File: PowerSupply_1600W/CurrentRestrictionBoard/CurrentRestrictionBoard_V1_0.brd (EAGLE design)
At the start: 160 x 100 mm, 0 parts

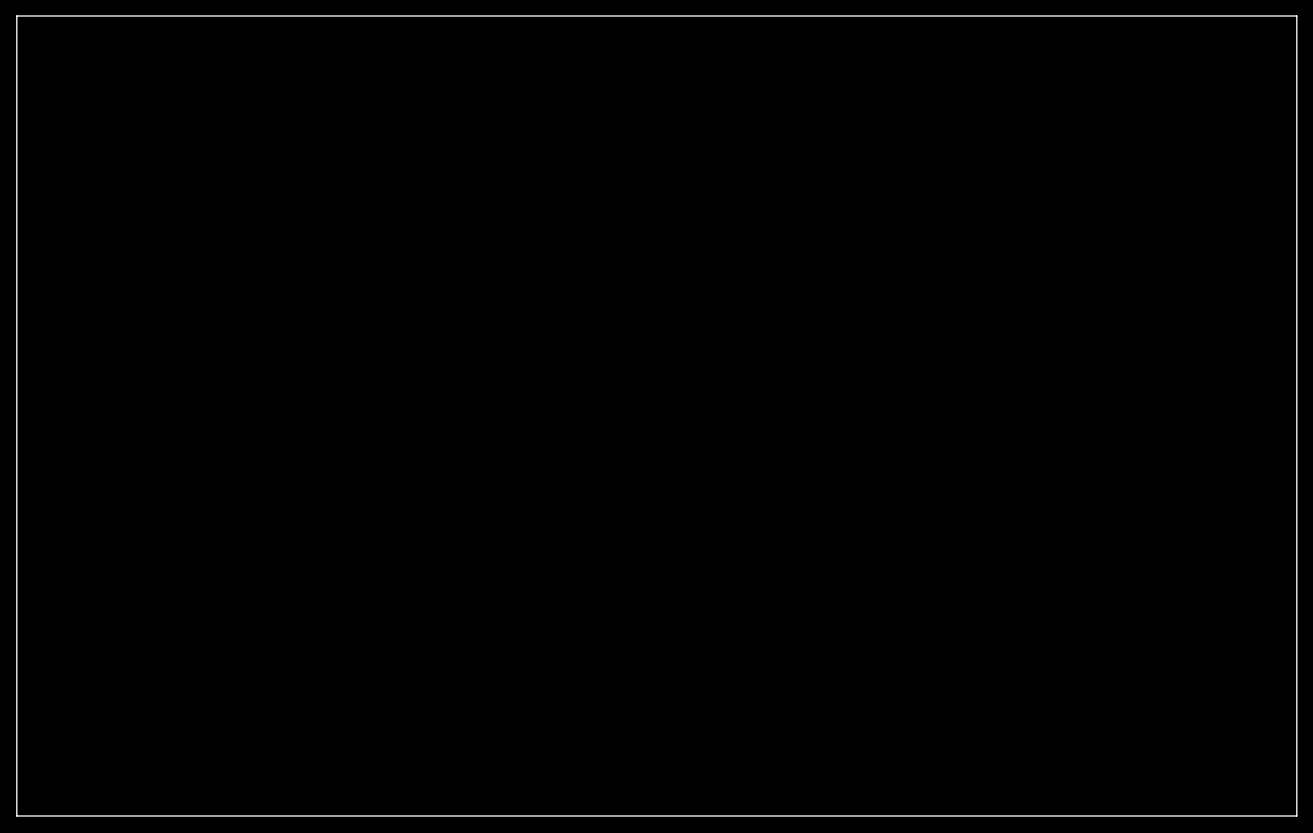
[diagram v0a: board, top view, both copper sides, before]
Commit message: PS 1600W Current restriction board.
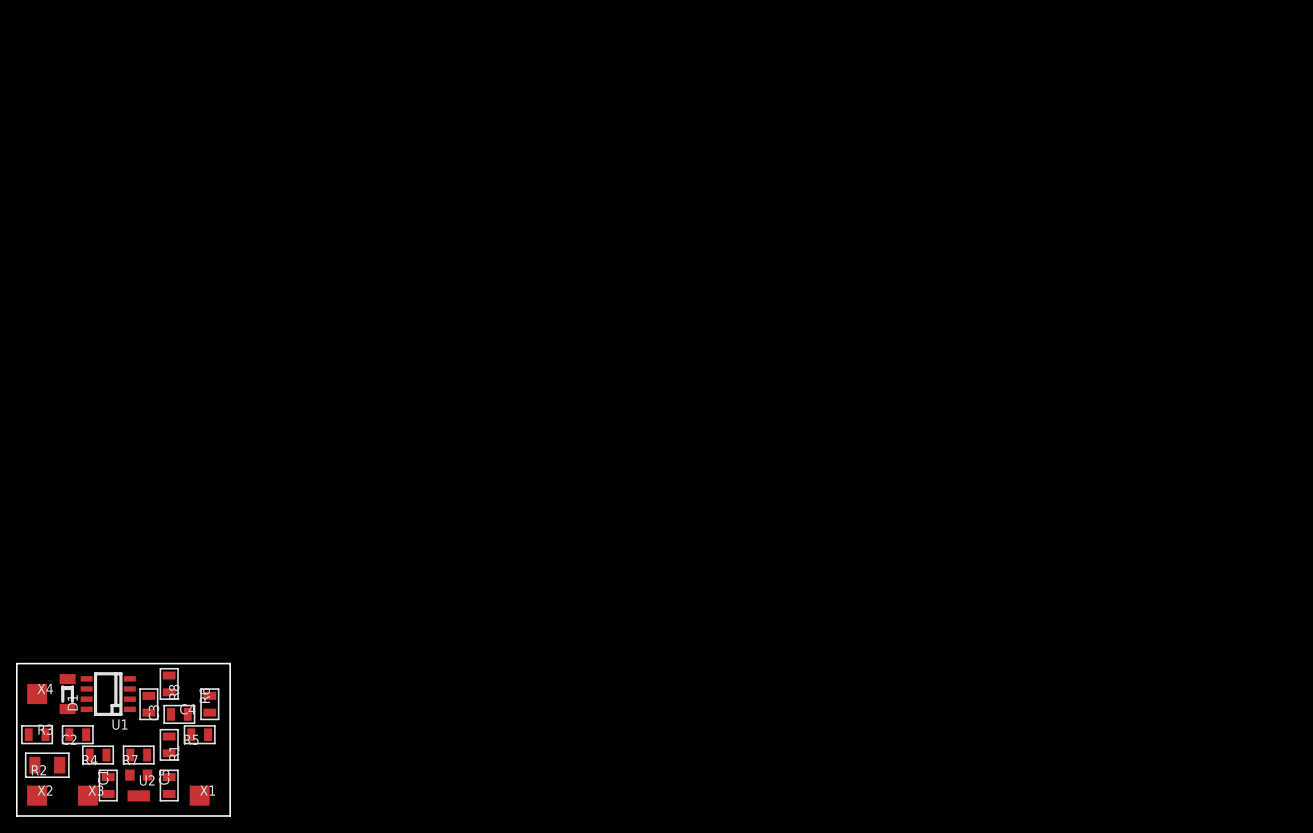
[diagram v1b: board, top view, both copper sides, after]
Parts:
- added C1, C4, R5: *, __MyCommonLib1:RSMD_0805
- added C2: 0.47uF x 16V, __MyCommonLib1:RSMD_0805
- added C3: 1n0 16V, __MyCommonLib1:RSMD_0805
- added C5: 0.1uF x 16V, __MyCommonLib1:RSMD_0805
- added D1: LL4148, __MyCommonLib1:SOD-80
- added R1: 22K, __MyCommonLib1:RSMD_0805
- added R2: 10R, __MyCommonLib1:RSMD_1206
- added R3, R7: 5K1, __MyCommonLib1:RSMD_0805
- added R4: RSMD_0805, __MyCommonLib1:RSMD_0805
- added R6: 680K, __MyCommonLib1:RSMD_0805
- added R8: 10K, __MyCommonLib1:RSMD_0805
- added U1: LM358, __MyCommonLib1:SOIC8
- added U2: TL431, __MyCommonLib1:SOT23
- added X1: GND, __MyCommonLib1:PIN1X1_2.5X2.5MM
- added X2: +12V, __MyCommonLib1:PIN1X1_2.5X2.5MM
- added X3: CS_IN, __MyCommonLib1:PIN1X1_2.5X2.5MM
- added X4: VReg_OUT, __MyCommonLib1:PIN1X1_2.5X2.5MM
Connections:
- new net +12V: C2.PAD_1, R2.PAD_0, R7.PAD_1, U1.8
- new net GND: C1.PAD_0, C2.PAD_0, C5.PAD_0, R8.PAD_0, U1.4, U2.3, X1.1
- new net N$1: R2.PAD_1, X2.1
- new net N$10: C5.PAD_1, R1.PAD_1, R7.PAD_0, U2.1, U2.2
- new net N$2: R4.PAD_1, X3.1
- new net N$3: C1.PAD_1, R4.PAD_0, U1.3
- new net N$4: C3.PAD_0, C4.PAD_0, R1.PAD_0, R6.PAD_1, R8.PAD_1, U1.2
- new net N$5: C3.PAD_1, R5.PAD_0, R6.PAD_0, U1.1, U1.5
- new net N$6: C4.PAD_1, R5.PAD_1
- new net N$7: D1.CATHODE, R3.PAD_1, U1.6
- new net N$8: D1.ANODE, U1.7
- new net N$9: R3.PAD_0, X4.1
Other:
- board size 160 x 100 mm -> 26.7 x 19.1 mm
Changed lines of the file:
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@@
 <setting verticaltext="up"/>
 </settings>
-<grid distance="0.05" unitdist="inch" unit="inch" style="lines" multiple="1" display="no" altdistance="0.025" altunitdist="inch" altunit="inch"/>
+<grid distance="0.05" unitdist="inch" unit="mm" style="lines" multiple="1" display="yes" altdistance="0.025" altunitdist="inch" altunit="inch"/>
 <layers>
 <layer number="1" name="Top" color="4" fill="1" visible="yes" active="yes"/>
@@
 <layer number="23" name="tOrigins" color="15" fill="1" visible="yes" active="yes"/>
 <layer number="24" name="bOrigins" color="15" fill="1" visible="yes" active="yes"/>
-<layer number="25" name="tNames" color="7" fill="1" visible="yes" active="yes"/>
-<layer number="26" name="bNames" color="7" fill="1" visible="yes" active="yes"/>
-<layer number="27" name="tValues" color="7" fill="1" visible="yes" active="yes"/>
-<layer number="28" name="bValues" color="7" fill="1" visible="yes" active="yes"/>
+<layer number="25" name="tNames" color="7" fill="1" visible="no" active="yes"/>
+<layer number="26" name="bNames" color="7" fill="1" visible="no" active="yes"/>
+<layer number="27" name="tValues" color="7" fill="1" visible="no" active="yes"/>
+<layer number="28" name="bValues" color="7" fill="1" visible="no" active="yes"/>
 <layer number="29" name="tStop" color="7" fill="3" visible="no" active="yes"/>
 <layer number="30" name="bStop" color="7" fill="6" visible="no" active="yes"/>
@@
 <board>
 <plain>
-<wire x1="0" y1="0" x2="160" y2="0" width="0" layer="20"/>
-<wire x1="160" y1="0" x2="160" y2="100" width="0" layer="20"/>
-<wire x1="160" y1="100" x2="0" y2="100" width="0" layer="20"/>
-<wire x1="0" y1="100" x2="0" y2="0" width="0" layer="20"/>
+<wire x1="0" y1="0" x2="26.67" y2="0" width="0.2" layer="20"/>
+<wire x1="26.67" y1="0" x2="26.67" y2="19.05" width="0.2" layer="20"/>
+<wire x1="26.67" y1="19.05" x2="0" y2="19.05" width="0.2" layer="20"/>
+<wire x1="0" y1="19.05" x2="0" y2="0" width="0.2" layer="20"/>
 </plain>
 <attributes>
@@
 </autorouter>
 <elements>
+<element name="U1" library="__MyCommonLib1" package="SOIC8" value="LM358" x="11.43" y="15.24" rot="R180"/>
+<element name="C1" library="__MyCommonLib1" package="RSMD_0805" value="*" x="11.43" y="3.81" rot="R90"/>
+<element name="D1" library="__MyCommonLib1" package="SOD-80" value="LL4148" x="6.35" y="15.24" rot="R270"/>
+<element name="R1" library="__MyCommonLib1" package="RSMD_0805" value="22K" x="19.05" y="8.89" rot="R270"/>
+<element name="U2" library="__MyCommonLib1" package="SOT23" value="TL431" x="15.24" y="3.81"/>
+<element name="X1" library="__MyCommonLib1" package="PIN1X1_2.5X2.5MM" value="GND" x="22.86" y="2.54"/>
+<element name="X2" library="__MyCommonLib1" package="PIN1X1_2.5X2.5MM" value="+12V" x="2.54" y="2.54"/>
+<element name="X3" library="__MyCommonLib1" package="PIN1X1_2.5X2.5MM" value="CS_IN" x="8.89" y="2.54"/>
+<element name="X4" library="__MyCommonLib1" package="PIN1X1_2.5X2.5MM" value="VReg_OUT" x="2.54" y="15.24"/>
+<element name="R2" library="__MyCommonLib1" package="RSMD_1206" value="10R" x="3.81" y="6.35" rot="R180"/>
+<element name="R3" library="__MyCommonLib1" package="RSMD_0805" value="5K1" x="2.54" y="10.16"/>
+<element name="C2" library="__MyCommonLib1" package="RSMD_0805" value="0.47uF x 16V" x="7.62" y="10.16" rot="R180"/>
+<element name="R4" library="__MyCommonLib1" package="RSMD_0805" value="RSMD_0805" x="10.16" y="7.62" rot="R180"/>
+<element name="C3" library="__MyCommonLib1" package="RSMD_0805" value="1n0 16V" x="16.51" y="13.97" rot="R270"/>
+<element name="C4" library="__MyCommonLib1" package="RSMD_0805" value="*" x="20.32" y="12.7"/>
+<element name="R5" library="__MyCommonLib1" package="RSMD_0805" value="*" x="22.86" y="10.16" rot="R180"/>
+<element name="R6" library="__MyCommonLib1" package="RSMD_0805" value="680K" x="24.13" y="13.97" rot="R90"/>
+<element name="C5" library="__MyCommonLib1" package="RSMD_0805" value="0.1uF x 16V" x="19.05" y="3.81" rot="R90"/>
+<element name="R7" library="__MyCommonLib1" package="RSMD_0805" value="5K1" x="15.24" y="7.62" rot="R180"/>
+<element name="R8" library="__MyCommonLib1" package="RSMD_0805" value="10K" x="19.05" y="16.51" rot="R270"/>
 </elements>
 <signals>
+<signal name="GND">
+<contactref element="U1" pad="4"/>
+<contactref element="X1" pad="1"/>
+<contactref element="C2" pad="PAD_0"/>
+<contactref element="U1" pad="4"/>
+<contactref element="C1" pad="PAD_0"/>
+<contactref element="U2" pad="3"/>
+<contactref element="C5" pad="PAD_0"/>
+<contactref element="R8" pad="PAD_0"/>
+<wire x1="14.12875" y1="17.145" x2="19.05" y2="17.56" width="0" layer="19" extent="1-1"/>
+<wire x1="8.67" y1="10.16" x2="14.12875" y2="17.145" width="0" layer="19" extent="1-1"/>
+<wire x1="11.43" y1="2.76" x2="8.67" y2="10.16" width="0" layer="19" extent="1-1"/>
+<wire x1="15.24" y1="2.51" x2="11.43" y2="2.76" width="0" layer="19" extent="1-1"/>
+<wire x1="19.05" y1="2.76" x2="15.24" y2="2.51" width="0" layer="19" extent="1-1"/>
+<wire x1="22.86" y1="2.54" x2="19.05" y2="2.76" width="0" layer="19" extent="1-1"/>
+</signal>
+<signal name="N$1">
+<contactref element="X2" pad="1"/>
+<contactref element="R2" pad="PAD_1"/>
+<wire x1="2.26" y1="6.35" x2="2.54" y2="2.54" width="0" layer="19" extent="1-1"/>
+</signal>
+<signal name="+12V">
+<contactref element="R2" pad="PAD_0"/>
+<contactref element="C2" pad="PAD_1"/>
+<contactref element="U1" pad="8"/>
+<contactref element="R7" pad="PAD_1"/>
+<wire x1="6.57" y1="10.16" x2="8.73125" y2="13.335" width="0" layer="19" extent="1-1"/>
+<wire x1="5.36" y1="6.35" x2="6.57" y2="10.16" width="0" layer="19" extent="1-1"/>
+<wire x1="14.19" y1="7.62" x2="8.73125" y2="13.335" width="0" layer="19" extent="1-1"/>
+</signal>
+<signal name="N$2">
+<contactref element="X3" pad="1"/>
+<contactref element="R4" pad="PAD_1"/>
+<wire x1="8.89" y1="2.54" x2="9.11" y2="7.62" width="0" layer="19" extent="1-1"/>
+</signal>
+<signal name="N$3">
+<contactref element="R4" pad="PAD_0"/>
+<contactref element="C1" pad="PAD_1"/>
+<contactref element="U1" pad="3"/>
+<wire x1="11.21" y1="7.62" x2="14.12875" y2="15.875" width="0" layer="19" extent="1-1"/>
+<wire x1="11.43" y1="4.86" x2="11.21" y2="7.62" width="0" layer="19" extent="1-1"/>
+</signal>
+<signal name="N$5">
+<contactref element="R6" pad="PAD_0"/>
+<contactref element="U1" pad="1"/>
+<contactref element="R5" pad="PAD_0"/>
+<contactref element="C3" pad="PAD_1"/>
+<contactref element="U1" pad="5"/>
+<wire x1="23.91" y1="10.16" x2="24.13" y2="12.92" width="0" layer="19" extent="1-1"/>
+<wire x1="16.51" y1="12.92" x2="24.13" y2="12.92" width="0" layer="19" extent="1-1"/>
+<wire x1="14.12875" y1="13.335" x2="16.51" y2="12.92" width="0" layer="19" extent="1-1"/>
+<wire x1="8.73125" y1="17.145" x2="14.12875" y2="13.335" width="0" layer="19" extent="1-1"/>
+</signal>
+<signal name="N$6">
+<contactref element="C4" pad="PAD_1"/>
+<contactref element="R5" pad="PAD_1"/>
+<wire x1="21.81" y1="10.16" x2="21.37" y2="12.7" width="0" layer="19" extent="1-1"/>
+</signal>
+<signal name="N$7">
+<contactref element="U1" pad="6"/>
+<contactref element="D1" pad="CATHODE"/>
+<contactref element="R3" pad="PAD_1"/>
+<wire x1="6.35" y1="17.115" x2="8.73125" y2="15.875" width="0" layer="19" extent="1-1"/>
+<wire x1="3.59" y1="10.16" x2="6.35" y2="17.115" width="0" layer="19" extent="1-1"/>
+</signal>
+<signal name="N$8">
+<contactref element="U1" pad="7"/>
+<contactref element="D1" pad="ANODE"/>
+<wire x1="6.35" y1="13.365" x2="8.73125" y2="14.605" width="0" layer="19" extent="1-1"/>
+</signal>
+<signal name="N$9">
+<contactref element="R3" pad="PAD_0"/>
+<contactref element="X4" pad="1"/>
+<wire x1="1.49" y1="10.16" x2="2.54" y2="15.24" width="0" layer="19" extent="1-1"/>
+</signal>
+<signal name="N$10">
+<contactref element="U2" pad="1"/>
+<contactref element="C5" pad="PAD_1"/>
+<contactref element="U2" pad="2"/>
+<contactref element="R7" pad="PAD_0"/>
+<contactref element="R1" pad="PAD_1"/>
+<wire x1="16.29" y1="7.62" x2="19.05" y2="7.84" width="0" layer="19" extent="1-1"/>
+<wire x1="16.34" y1="5.11" x2="16.29" y2="7.62" width="0" layer="19" extent="1-1"/>
+<wire x1="14.14" y1="5.11" x2="16.34" y2="5.11" width="0" layer="19" extent="1-1"/>
+<wire x1="19.05" y1="4.86" x2="16.34" y2="5.11" width="0" layer="19" extent="1-1"/>
+</signal>
+<signal name="N$4">
+<contactref element="R8" pad="PAD_1"/>
+<contactref element="R1" pad="PAD_0"/>
+<contactref element="R6" pad="PAD_1"/>
+<contactref element="U1" pad="2"/>
+<contactref element="C3" pad="PAD_0"/>
+<contactref element="C4" pad="PAD_0"/>
+<wire x1="19.05" y1="15.46" x2="24.13" y2="15.02" width="0" layer="19" extent="1-1"/>
+<wire x1="16.51" y1="15.02" x2="19.05" y2="15.46" width="0" layer="19" extent="1-1"/>
+<wire x1="14.12875" y1="14.605" x2="16.51" y2="15.02" width="0" layer="19" extent="1-1"/>
+<wire x1="19.27" y1="12.7" x2="19.05" y2="15.46" width="0" layer="19" extent="1-1"/>
+<wire x1="19.05" y1="9.94" x2="19.27" y2="12.7" width="0" layer="19" extent="1-1"/>
+</signal>
 </signals>
 </board>
